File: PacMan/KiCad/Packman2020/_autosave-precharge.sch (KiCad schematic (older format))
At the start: 17 parts, among them J1 DF22-1P-7.92DSA(05), J2 DF22-1P-7.92DSA(05), J3 DF22-1P-7.92DSA(05), J4 JST PH, K1 G2RL, K2 G5V-1, Q1 MMBT2222A

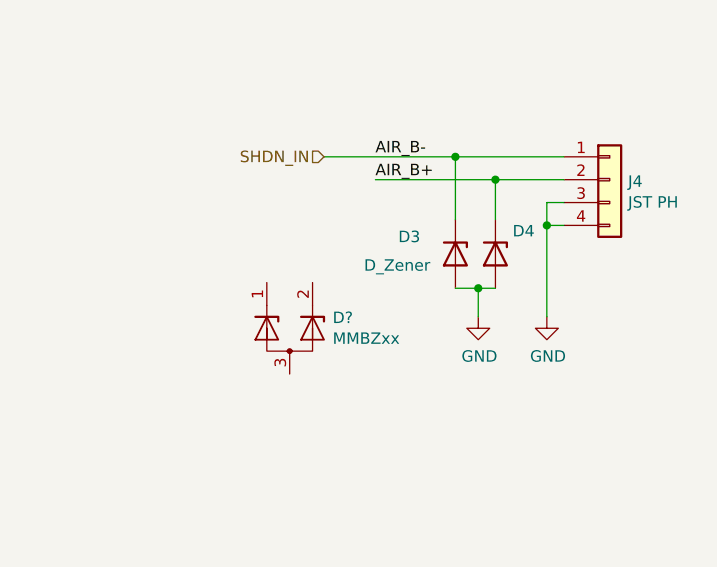
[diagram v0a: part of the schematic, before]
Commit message: PacMan initial commit
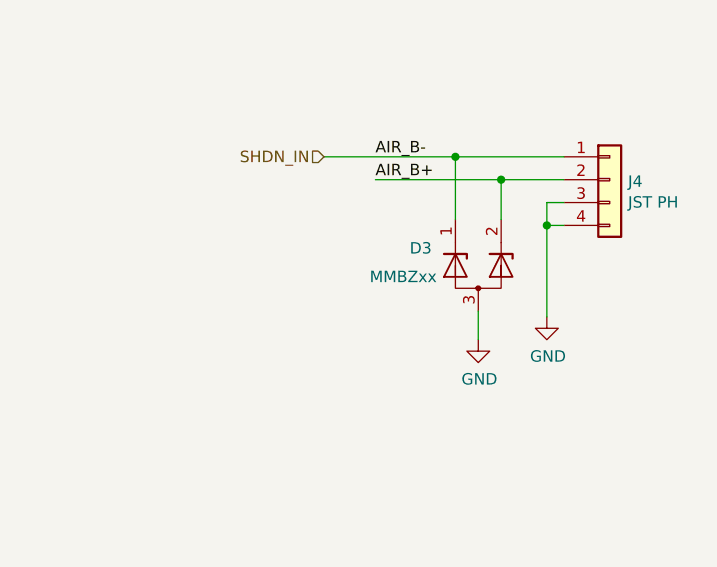
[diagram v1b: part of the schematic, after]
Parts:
- removed D3, D4: D_Zener, Diode_SMD:D_SMB_Handsoldering, symbol Device:D_Zener
- D3: renamed from D?; footprint Package_TO_SOT_SMD:SOT-23 -> Package_TO_SOT_SMD:SOT-23_Handsoldering
- Q1: footprint DigiKey_Lib:SOT-23-3 -> Package_TO_SOT_SMD:SOT-23
- R1, R2, R3: footprint Resistor_SMD:R_0603_1608Metric_Pad1.05x0.95mm_HandSolder -> Resistor_SMD:R_0603_1608Metric_Pad0.98x0.95mm_HandSolder
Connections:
- net AIR_B+: now also D3.2 (K)
- net GND: now also D3.3 (A)
- net SHDN_IN: now also D3.1 (K)
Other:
- moved on the sheet: D3
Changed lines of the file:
@@
 F 0 "R1" V 3293 3450 50  0000 C CNN
 F 1 "R" V 3384 3450 50  0000 C CNN
-F 2 "Resistor_SMD:R_0603_1608Metric_Pad1.05x0.95mm_HandSolder" V 3430 3450 50  0001 C CNN
+F 2 "Resistor_SMD:R_0603_1608Metric_Pad0.98x0.95mm_HandSolder" V 3430 3450 50  0001 C CNN
 F 3 "~" H 3500 3450 50  0001 C CNN
 	1    3500 3450
@@
 F 0 "Q1" H 4616 3696 50  0000 L CNN
 F 1 "MMBT2222A" H 4616 3605 50  0000 L CNN
-F 2 "DigiKey_Lib:SOT-23-3" H 4625 3750 50  0001 C CNN
+F 2 "Package_TO_SOT_SMD:SOT-23" H 4625 3750 50  0001 C CNN
 F 3 "~" H 4425 3650 50  0001 C CNN
 	1    4425 3650
@@
 F 0 "R2" V 4568 3650 50  0000 C CNN
 F 1 "R" V 4659 3650 50  0000 C CNN
-F 2 "Resistor_SMD:R_0603_1608Metric_Pad1.05x0.95mm_HandSolder" V 4705 3650 50  0001 C CNN
+F 2 "Resistor_SMD:R_0603_1608Metric_Pad0.98x0.95mm_HandSolder" V 4705 3650 50  0001 C CNN
 F 3 "~" H 4775 3650 50  0001 C CNN
 	1    4775 3650
@@
 F 0 "R3" H 4995 4046 50  0000 L CNN
 F 1 "R" H 4995 3955 50  0000 L CNN
-F 2 "Resistor_SMD:R_0603_1608Metric_Pad1.05x0.95mm_HandSolder" V 4855 4000 50  0001 C CNN
+F 2 "Resistor_SMD:R_0603_1608Metric_Pad0.98x0.95mm_HandSolder" V 4855 4000 50  0001 C CNN
 F 3 "~" H 4925 4000 50  0001 C CNN
 	1    4925 4000
@@
 	7575 2675 8150 2675
 Wire Wire Line
-	7800 2775 8325 2775
-$Comp
-L Device:D_Zener D3
-U 1 1 5FAA05CE
-P 8150 3100
-F 0 "D3" V 8075 2850 50  0000 L CNN
-F 1 "D_Zener" V 8200 2700 50  0000 L CNN
-F 2 "Diode_SMD:D_SMB_Handsoldering" H 8150 3100 50  0001 C CNN
-F 3 "~" H 8150 3100 50  0001 C CNN
-	1    8150 3100
-	0    1    1    0
-$EndComp
-$Comp
-L Device:D_Zener D4
-U 1 1 5FAA0C74
-P 8325 3100
-F 0 "D4" V 8225 3175 50  0000 L CNN
-F 1 "D_Zener" V 8375 2700 50  0001 L CNN
-F 2 "Diode_SMD:D_SMB_Handsoldering" H 8325 3100 50  0001 C CNN
-F 3 "~" H 8325 3100 50  0001 C CNN
-	1    8325 3100
-	0    1    1    0
-$EndComp
+	7800 2775 8350 2775
 Wire Wire Line
 	8625 2875 8550 2875
@@
 L power:GND #PWR0102
 U 1 1 5FAA23F0
-P 8250 3375
-F 0 "#PWR0102" H 8250 3125 50  0001 C CNN
-F 1 "GND" H 8255 3202 50  0000 C CNN
-F 2 "" H 8250 3375 50  0001 C CNN
-F 3 "" H 8250 3375 50  0001 C CNN
-	1    8250 3375
+P 8250 3475
+F 0 "#PWR0102" H 8250 3225 50  0001 C CNN
+F 1 "GND" H 8255 3302 50  0000 C CNN
+F 2 "" H 8250 3475 50  0001 C CNN
+F 3 "" H 8250 3475 50  0001 C CNN
+	1    8250 3475
 	1    0    0    -1
 $EndComp
@@
 Connection ~ 8550 2975
 Wire Wire Line
-	8250 3375 8250 3250
-Wire Wire Line
-	8250 3250 8325 3250
-Wire Wire Line
-	8250 3250 8150 3250
-Connection ~ 8250 3250
+	8250 3475 8250 3350
 Wire Wire Line
 	8150 2950 8150 2675
@@
 	8150 2675 8625 2675
 Wire Wire Line
-	8325 2950 8325 2775
-Connection ~ 8325 2775
-Wire Wire Line
-	8325 2775 8625 2775
+	8350 2950 8350 2775
+Connection ~ 8350 2775
+Wire Wire Line
+	8350 2775 8625 2775
 Wire Wire Line
 	5050 5150 5050 5500
 $Comp
-L Diode:MMBZxx D?
+L Diode:MMBZxx D3
 U 1 1 601F4E4A
-P 7425 3425
-F 0 "D?" H 7613 3471 50  0000 L CNN
-F 1 "MMBZxx" H 7613 3380 50  0000 L CNN
-F 2 "Package_TO_SOT_SMD:SOT-23" H 7575 3325 50  0001 L CNN
-F 3 "http://www.onsemi.com/pub/Collateral/MMBZ5V6ALT1-D.PDF" V 7325 3425 50  0001 C CNN
-	1    7425 3425
-	1    0    0    -1
-$EndComp
+P 8250 3150
+F 0 "D3" H 7950 3225 50  0000 L CNN
+F 1 "MMBZxx" H 7775 3100 50  0000 L CNN
+F 2 "Package_TO_SOT_SMD:SOT-23_Handsoldering" H 8400 3050 50  0001 L CNN
+F 3 "http://www.onsemi.com/pub/Collateral/MMBZ5V6ALT1-D.PDF" V 8150 3150 50  0001 C CNN
+	1    8250 3150
+	1    0    0    -1
+$EndComp
